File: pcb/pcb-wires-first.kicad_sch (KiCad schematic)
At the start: 13 parts, among them J1 Conn_01x06, J2 Conn_01x02, J3 Conn_01x04, J4 Conn_01x06, SW1 SW_Push, SW2 SW_Push, U1 SLG47115V

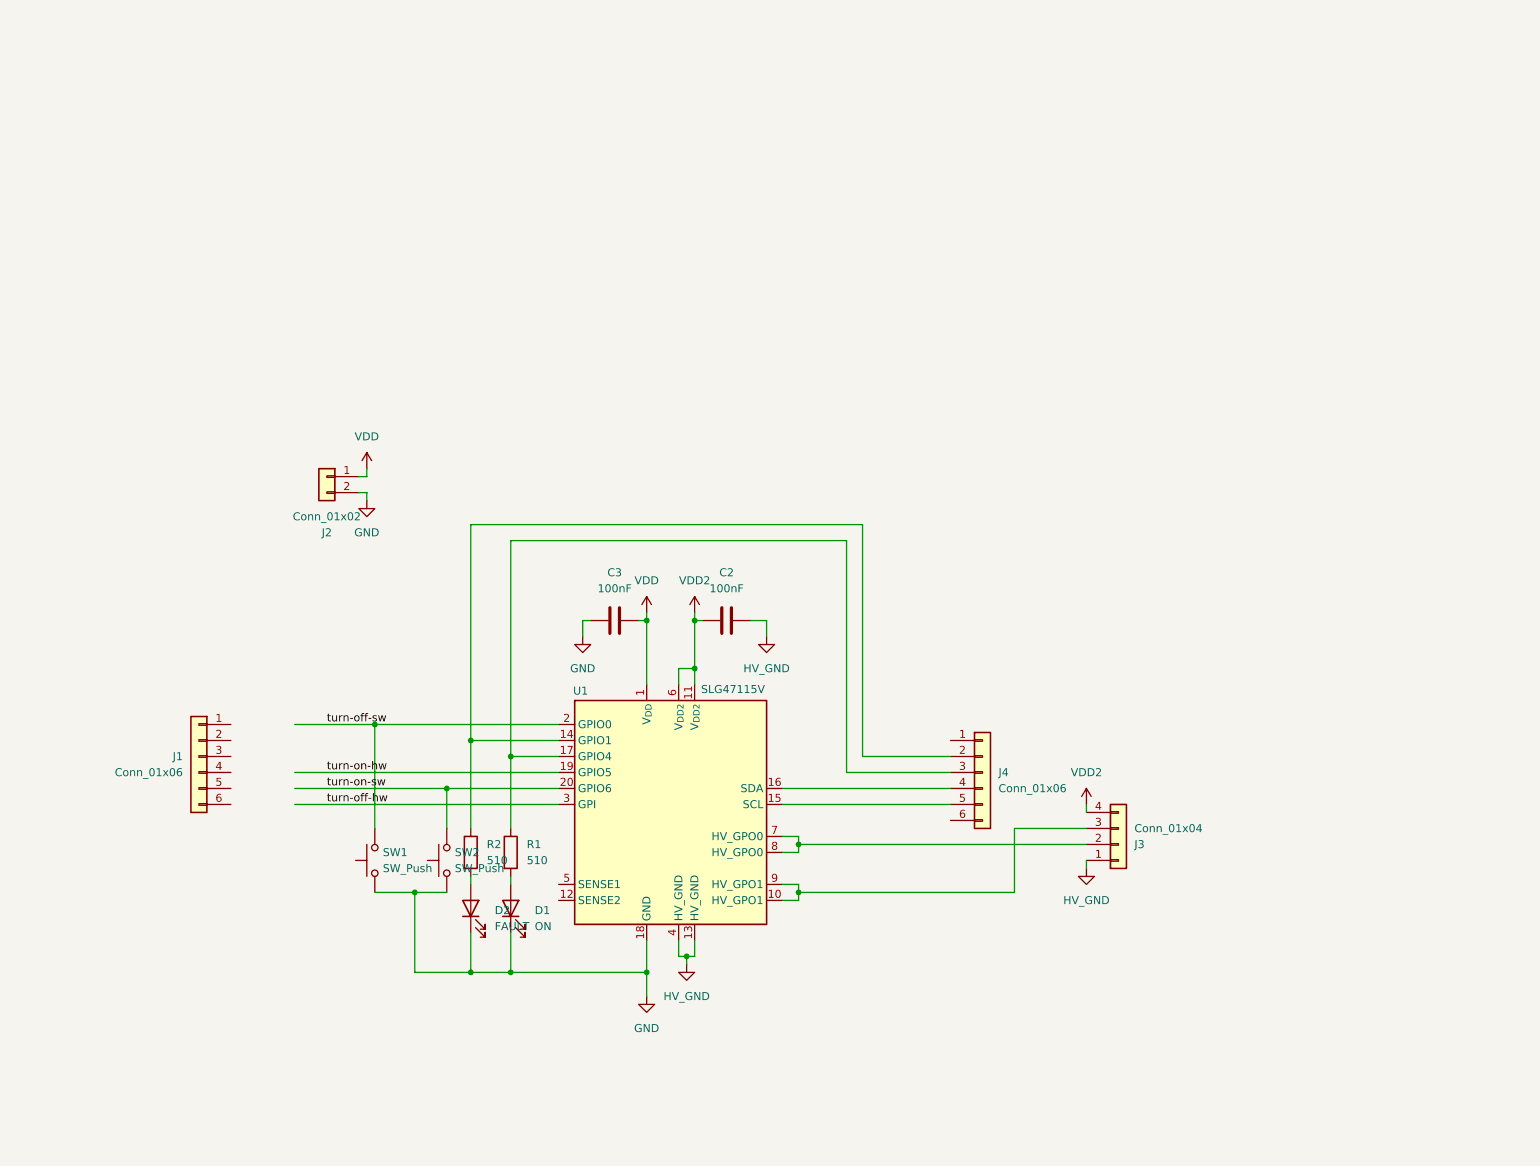
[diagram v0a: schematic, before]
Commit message: Drafting the board.
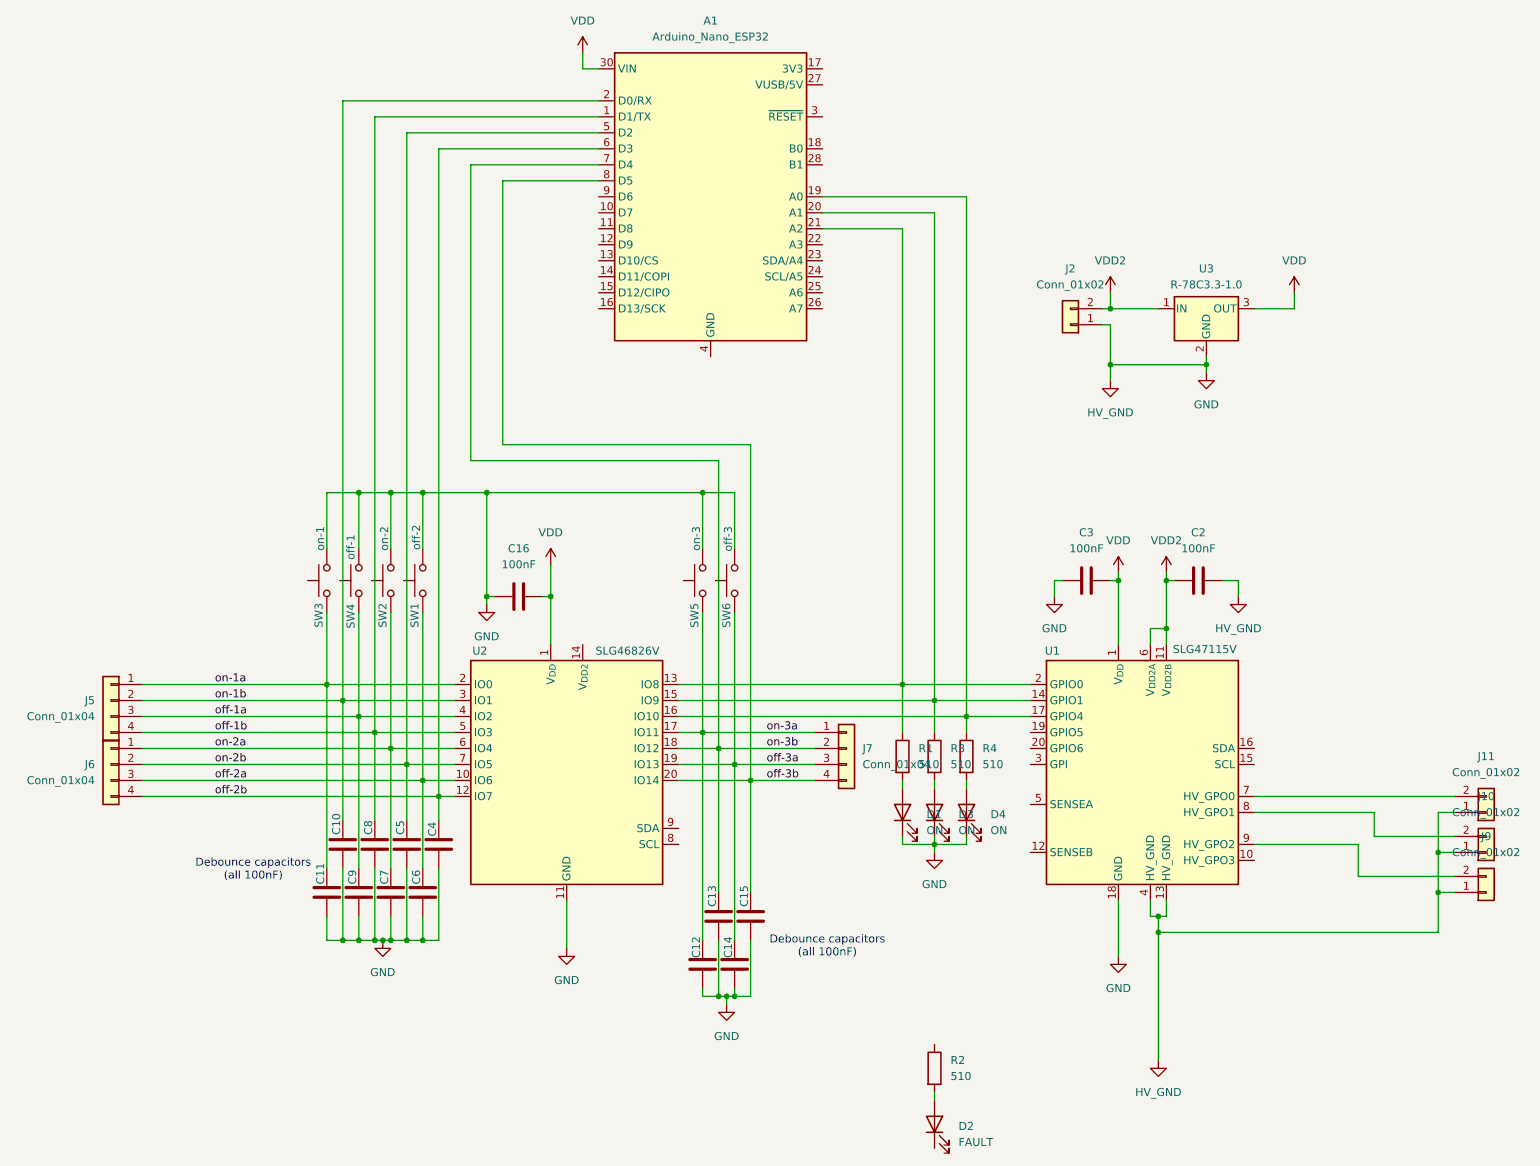
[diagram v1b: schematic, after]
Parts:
- removed J1: Conn_01x06, symbol Connector_Generic:Conn_01x06
- removed J3: Conn_01x04, Connector_PinHeader_2.54mm:PinHeader_1x04_P2.54mm_Vertical, symbol Connector_Generic:Conn_01x04
- removed J4: Conn_01x06, Connector_PinHeader_2.54mm:PinHeader_1x06_P2.54mm_Vertical, symbol Connector_Generic:Conn_01x06
- added A1: Arduino_Nano_ESP32, Module:Arduino_Nano, symbol MCU_Module:Arduino_Nano_ESP32
- added C10, C11, C12, C13, C14, C15, C16, C4, C5, C6, C7, C8, C9: 100nF, Capacitor_SMD:C_0603_1608Metric, symbol Device:C
- added D3, D4: ON, Diode_SMD:D_0603_1608Metric, symbol Device:LED
- added J10, J11, J9: Conn_01x02, Connector_Phoenix_MC:PhoenixContact_MCV_1,5_2-G-3.5_1x02_P3.50mm_Vertical, symbol Connector_Generic:Conn_01x02
- added J5, J6, J7: Conn_01x04, Connector_Phoenix_MC:PhoenixContact_MCV_1,5_4-G-3.5_1x04_P3.50mm_Vertical, symbol Connector_Generic:Conn_01x04
- added R3, R4: 510, Resistor_SMD:R_0603_1608Metric, symbol Device:R
- added SW3: on-1, Button_Switch_SMD:SW_SPST_B3U-1000P, symbol Switch:SW_Push
- added SW4: off-1, Button_Switch_SMD:SW_SPST_B3U-1000P, symbol Switch:SW_Push
- added SW5: on-3, Button_Switch_SMD:SW_SPST_B3U-1000P, symbol Switch:SW_Push
- added SW6: off-3, Button_Switch_SMD:SW_SPST_B3U-1000P, symbol Switch:SW_Push
- added U2: SLG46826V, Package_DFN_QFN:Renesas_UQFN-20_2x3mm_P0.4mm_LayoutBorder4x6y, symbol local-lib:SLG46826V
- added U3: R-78C3.3-1.0, Converter_DCDC:Converter_DCDC_RECOM_R-78E-0.5_THT, symbol Converter_DCDC:R-78C3.3-1.0
- J2: footprint (none) -> Connector_Phoenix_MSTB:PhoenixContact_MSTBVA_2,5_2-G-5,08_1x02_P5.08mm_Vertical
- SW1: value SW_Push -> off-2
- SW2: value SW_Push -> on-2
- U1: symbol local-lib:SLG47115V -> local-lib:SLG47105V
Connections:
- net HV_GND is gone; now on net GND: C2.1, U1.13 (HV_GND), U1.4 (HV_GND)
- net GND: now also J2.1 (Pin_1), SW1.2, SW2.2, C10.1, C11.1, C12.1, C13.1, C14.1, C15.1, C16.1, C4.1, C5.1, C6.1, C7.1, C8.1, C9.1, D3.1 (K), D4.1 (K), J10.1 (Pin_1), J11.1 (Pin_1), J9.1 (Pin_1), SW3.2, SW4.2, SW5.2, SW6.2, U2.11 (GND), U3.2 (GND); no longer D2.1 (K), J2.2 (Pin_2), SW1.1, SW2.1
- net VDD: now also A1.30 (VIN), C16.2, U2.1 (V_{DD}), U3.3 (OUT); no longer J2.1 (Pin_1)
- net VDD2: now also J2.2 (Pin_2), U3.1 (IN)
- net at U1.17 (GPIO4): now also A1.19 (A0), R4.1, U2.16 (IO10); no longer R1.1
- net at U1.14 (GPIO1): now also A1.20 (A1), R3.1, U2.15 (IO9); no longer R2.1
- net at U1.7 (HV_GPO0): now also J11.2 (Pin_2); no longer U1.8 (HV_GPO0)
- net at U1.9 (HV_GPO2): now also J9.2 (Pin_2); no longer U1.10 (HV_GPO1)
- net turn-off-hw: no longer names the net of U1.3 (GPI)
- net turn-off-sw: no longer names the net of U1.2 (GPIO0)
- net turn-off-sw: now also R1.1, A1.21 (A2), U2.13 (IO8); no longer SW1.2
- net turn-on-hw: no longer names the net of U1.19 (GPIO5)
- net turn-on-sw: no longer names the net of U1.20 (GPIO6)
- net turn-on-sw: no longer SW2.2
- new net: A1.29 (GND), A1.4 (GND)
- new net: D3.2 (A), R3.2
- new net: D4.2 (A), R4.2
- new net: J10.2 (Pin_2), U1.8 (HV_GPO1)
- new net off-1a: C9.2, J5.3 (Pin_3), SW4.1, U2.4 (IO2)
- new net off-1b: A1.1 (D1/TX), C8.2, J5.4 (Pin_4), U2.5 (IO3)
- new net off-2a: C6.2, J6.3 (Pin_3), SW1.1, U2.10 (IO6)
- new net off-2b: A1.6 (D3), C4.2, J6.4 (Pin_4), U2.12 (IO7)
- new net off-3a: C14.2, J7.3 (Pin_3), SW6.1, U2.19 (IO13)
- new net off-3b: A1.8 (D5), C15.2, J7.4 (Pin_4), U2.20 (IO14)
- new net on-1a: C11.2, J5.1 (Pin_1), SW3.1, U2.2 (IO0)
- new net on-1b: A1.2 (D0/RX), C10.2, J5.2 (Pin_2), U2.3 (IO1)
- new net on-2a: C7.2, J6.1 (Pin_1), SW2.1, U2.6 (IO4)
- new net on-2b: A1.5 (D2), C5.2, J6.2 (Pin_2), U2.7 (IO5)
- new net on-3a: C12.2, J7.1 (Pin_1), SW5.1, U2.17 (IO11)
- new net on-3b: A1.7 (D4), C13.2, J7.2 (Pin_2), U2.18 (IO12)
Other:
- note added: "Debounce capacitors (all 100nF)"
- moved on the sheet: C2, C3, D1, D2, J2, R1, R2, SW1, SW2, U1
